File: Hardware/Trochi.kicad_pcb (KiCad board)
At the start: 2 copper layers, 18.5 x 25 mm, 51 parts, among them IC1 ICM-42688-P, J1 JST-SH, J2 JST-SH, J3 JST PH, J6 JST-SH, J7 JST-SH, Q1 AO3400A, Q2 AO3400A, Q3 AO3400A, Q4 AO3400A, Q5 AO3400A, U1 ME6211C33M5, U3 YX-SMD5020

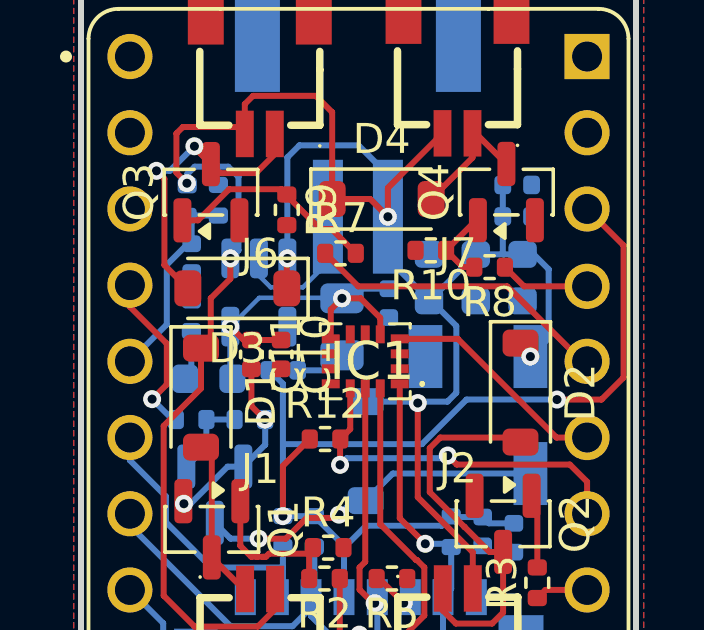
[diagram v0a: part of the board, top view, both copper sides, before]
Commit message: chore: snapshot PCB state before full re-layout
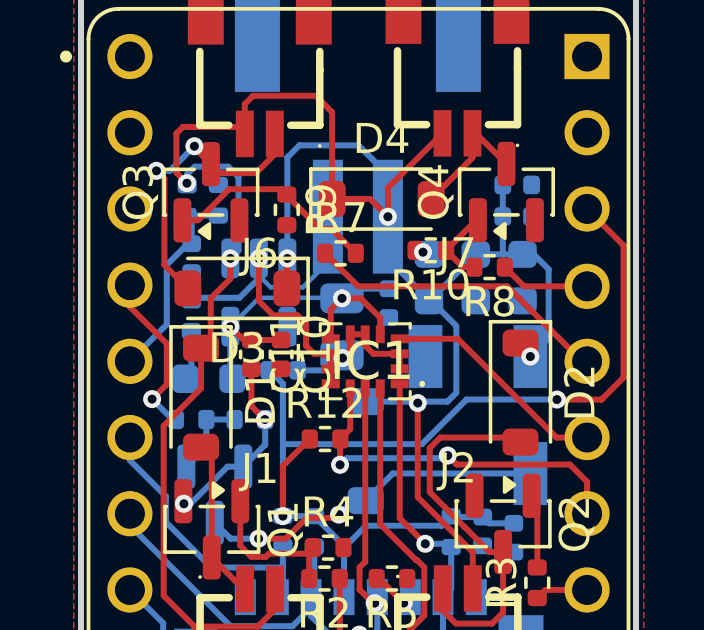
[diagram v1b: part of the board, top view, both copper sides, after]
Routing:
- net GND: track 15.0 -> 28.0 mm, vias 3 -> 6
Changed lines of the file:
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@@
 		(embedded_fonts no)
 		(model "C:/Users/husey/OneDrive/Belgeler/Trochi/Libraries/3D_Models/esp32_s3_supermini.step"
-			(opacity 0.0000)
 			(offset
 				(xyz 0 0 17.5)
@@
 	)
 	(segment
+		(start 139.76 104.33)
+		(end 138.956304 104.33)
+		(width 0.2)
+		(layer "F.Cu")
+		(net "GND")
+	)
+	(segment
+		(start 140.87 105.61)
+		(end 140.32 105.61)
+		(width 0.2)
+		(layer "F.Cu")
+		(net "GND")
+	)
+	(segment
 		(start 142.480947 113.1)
 		(end 143.300947 113.92)
@@
 	)
 	(segment
+		(start 140.87 106.11)
+		(end 140.87 106.61)
+		(width 0.2)
+		(layer "F.Cu")
+		(net "GND")
+	)
+	(segment
+		(start 142.29 105.61)
+		(end 142.02 105.34)
+		(width 0.2)
+		(layer "F.Cu")
+		(net "GND")
+	)
+	(segment
+		(start 143.17 105.61)
+		(end 143.17 106.11)
+		(width 0.2)
+		(layer "F.Cu")
+		(net "GND")
+	)
+	(segment
+		(start 140.32 105.61)
+		(end 140.05 105.34)
+		(width 0.2)
+		(layer "F.Cu")
+		(net "GND")
+	)
+	(segment
 		(start 142.4 113.1)
 		(end 142.480947 113.1)
@@
 	)
 	(segment
+		(start 142.02 104.96)
+		(end 141.52 104.96)
+		(width 0.2)
+		(layer "F.Cu")
+		(net "GND")
+	)
+	(segment
+		(start 140.05 105.34)
+		(end 140.05 104.62)
+		(width 0.2)
+		(layer "F.Cu")
+		(net "GND")
+	)
+	(segment
+		(start 143.17 105.61)
+		(end 142.29 105.61)
+		(width 0.2)
+		(layer "F.Cu")
+		(net "GND")
+	)
+	(segment
+		(start 143.945 102.220865)
+		(end 143.884135 102.16)
+		(width 0.2)
+		(layer "F.Cu")
+		(net "GND")
+	)
+	(segment
+		(start 141.52 105.493583)
+		(end 141.262145 105.751438)
+		(width 0.2)
+		(layer "F.Cu")
+		(net "GND")
+	)
+	(segment
+		(start 140.87 105.61)
+		(end 140.87 106.11)
+		(width 0.2)
+		(layer "F.Cu")
+		(net "GND")
+	)
+	(segment
+		(start 138.956304 104.33)
+		(end 138.475 103.848696)
+		(width 0.2)
+		(layer "F.Cu")
+		(net "GND")
+	)
+	(segment
+		(start 138.475 103.848696)
+		(end 138.475 102.43)
+		(width 0.2)
+		(layer "F.Cu")
+		(net "GND")
+	)
+	(segment
 		(start 138.225 106.11)
 		(end 138.225 107.35)
@@
 	)
 	(segment
+		(start 143.884135 102.16)
+		(end 143.695 102.16)
+		(width 0.2)
+		(layer "F.Cu")
+		(net "GND")
+	)
+	(segment
+		(start 140.05 104.62)
+		(end 139.76 104.33)
+		(width 0.2)
+		(layer "F.Cu")
+		(net "GND")
+	)
+	(segment
 		(start 138.225 107.35)
 		(end 138.675 107.8)
@@
 		(net "GND")
 	)
+	(segment
+		(start 141.52 104.96)
+		(end 141.52 105.493583)
+		(width 0.2)
+		(layer "F.Cu")
+		(net "GND")
+	)
+	(segment
+		(start 142.02 105.34)
+		(end 142.02 104.96)
+		(width 0.2)
+		(layer "F.Cu")
+		(net "GND")
+	)
 	(via
 		(at 138.675 107.8)
@@
 		(net "GND")
 	)
+	(via
+		(at 141.262145 105.751438)
+		(size 0.6)
+		(drill 0.3)
+		(layers "F.Cu" "B.Cu")
+		(net "GND")
+	)
+	(via
+		(at 143.945 102.220865)
+		(size 0.6)
+		(drill 0.3)
+		(layers "F.Cu" "B.Cu")
+		(net "GND")
+	)
+	(via
+		(at 138.475 102.43)
+		(size 0.6)
+		(drill 0.3)
+		(layers "F.Cu" "B.Cu")
+		(net "GND")
+	)
 	(segment
 		(start 140.895 101.19)
@@
 	)
 	(segment
+		(start 138.475 103.092499)
+		(end 138.475 102.43)
+		(width 0.2)
+		(layer "B.Cu")
+		(net "GND")
+	)
+	(segment
 		(start 140.745 106.16)
 		(end 141.245 105.66)
@@
 	)
 	(segment
+		(start 136.225 103.83)
+		(end 136.3125 103.7425)
+		(width 0.2)
+		(layer "B.Cu")
+		(net "GND")
+	)
+	(segment
 		(start 139.9425 103.3925)
 		(end 138.8675 103.3925)
@@
 	)
 	(segment
+		(start 137.824999 103.7425)
+		(end 138.475 103.092499)
+		(width 0.2)
+		(layer "B.Cu")
+		(net "GND")
+	)
+	(segment
 		(start 136.235 103.82)
 		(end 136.225 103.83)
@@
 	)
 	(segment
+		(start 136.3125 103.7425)
+		(end 137.824999 103.7425)
+		(width 0.2)
+		(layer "B.Cu")
+		(net "GND")
+	)
+	(segment
 		(start 138.685 107.8)
 		(end 138.685 108.64)
@@
 		(hatch edge 0.5)
 		(connect_pads
-			(clearance 0.3)
+			(clearance 0.2)
 		)
 		(min_thickness 0.25)

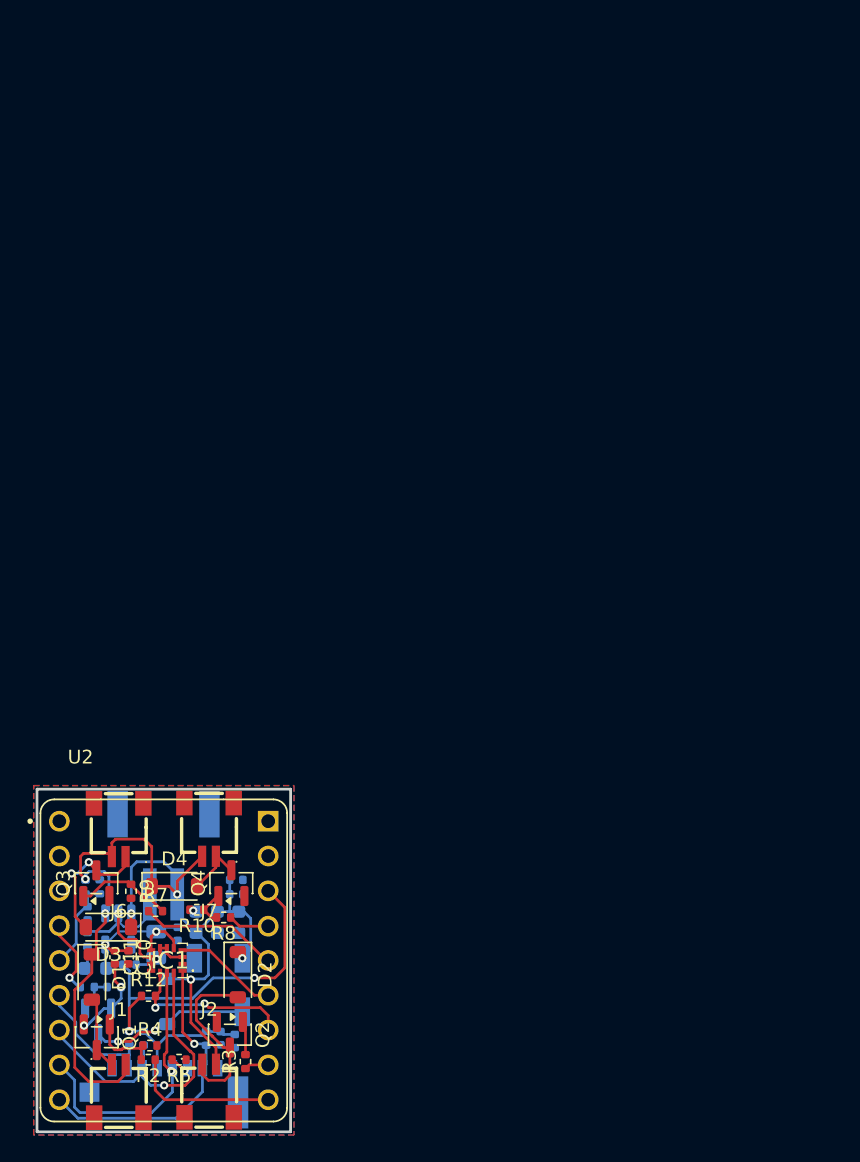
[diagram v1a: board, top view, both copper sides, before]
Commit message: feat: Routing Completed :)
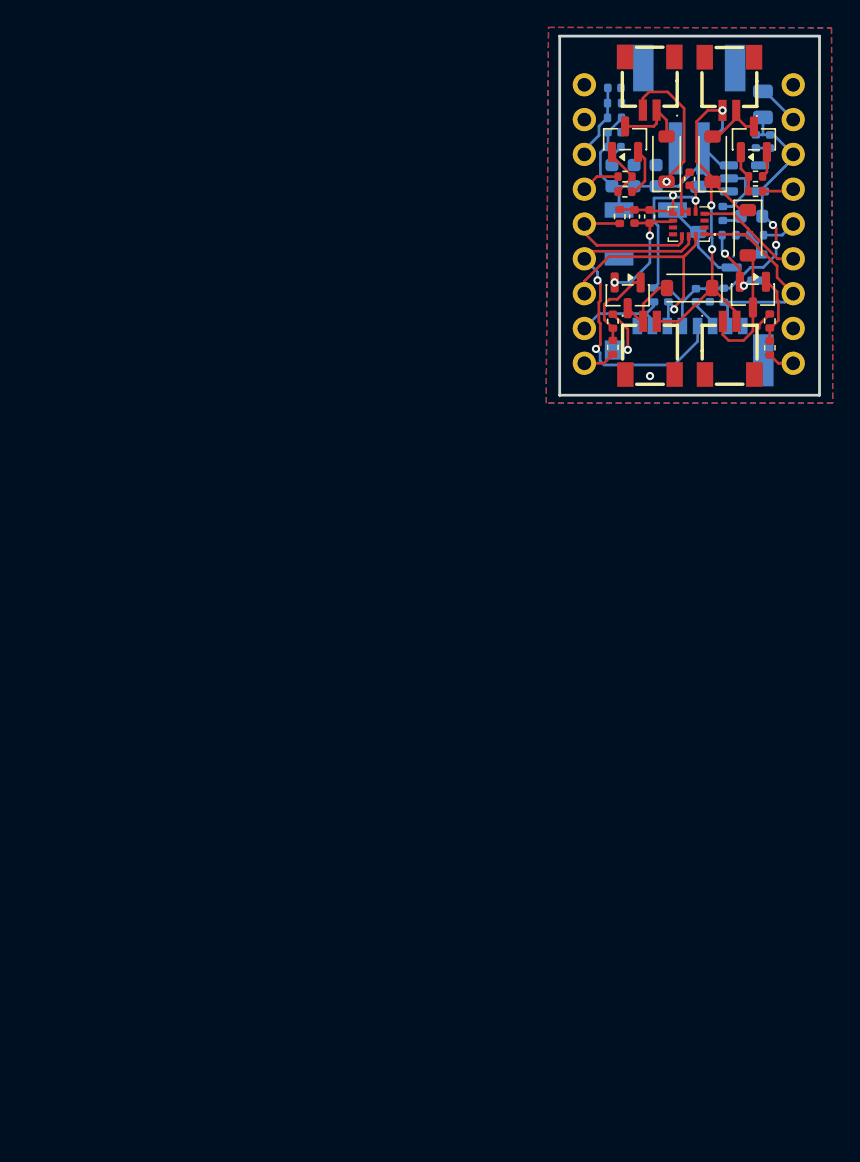
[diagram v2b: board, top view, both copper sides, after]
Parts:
- removed U2: ~, trochi_footprint:esp32_s3_supermini
- added C14: 10nF, Capacitor_SMD:C_0402_1005Metric, F.Cu at (176.1, 51.6)
- added J4: Conn_01x09, Connector_PinHeader_2.54mm:PinHeader_1x09_P2.54mm_Vertical, F.Cu at (172.5, 42.0)
- added J5: Conn_01x09, Connector_PinHeader_2.54mm:PinHeader_1x09_P2.54mm_Vertical, F.Cu at (187.7, 42.0)
- C11: value 100nF -> 2.2uF
- moved C6 75.6 mm to (185.5, 43.4), turned to 90 degrees
- moved C7 75.5 mm to (185.0, 46.1), turned to -90 degrees
- moved R16 73.4 mm to (185.0, 52.9), turned to 180 degrees
- moved D5 72.8 mm to (184.7, 51.6)
- moved Q5 72.5 mm to (184.2, 55.3), turned to 180 degrees
- moved C8 72.2 mm to (186.0, 46.1)
- moved C9 71.4 mm to (174.7, 42.2), turned to 0 degrees
- moved U1 71.3 mm to (184.2, 48.8), turned to 0 degrees
- moved R17 70.9 mm to (183.0, 52.9), turned to 180 degrees
- moved R11 70.4 mm to (182.6, 51.4)
- moved C10 70.0 mm to (180.2, 48.8)
- moved D6 69.6 mm to (180.8, 51.1)
- moved D3 69.3 mm to (178.5, 47.4), turned to 90 degrees
- moved R5 69.0 mm to (186.0, 59.2), turned to 90 degrees
- moved R6 68.4 mm to (174.7, 43.3), turned to 0 degrees
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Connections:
- C10 pad 1: +3.3V -> GND
- C10 pad 2: GND -> +3.3V
- C11 pad 1: +3.3V -> GND
- C11 pad 2: GND -> +3.3V
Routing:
- net GND: track 28.0 -> 41.2 mm
- net /VBAT: track 77.0 -> 68.4 mm, vias 6 -> 4
- net +3.3V: track 51.4 -> 43.6 mm
- net PWM_M1: track 10.8 -> 3.03 mm
- net PWM_M3: track 10.2 -> 2.84 mm
- net SPI_MISO: track 21.9 -> 15.9 mm, vias 1 -> 0
- net SPI_SCK: track 20.7 -> 26.3 mm, vias 1 -> 2
- net Net-(D6-A): track 11.6 -> 6.70 mm, vias 2 -> 0
- net SPI_MOSI: track 23.3 -> 18.4 mm
- net Net-(D3-A): track 9.97 -> 5.58 mm, vias 2 -> 0
- net Net-(D2-A): track 13.1 -> 9.32 mm
- net Net-(Q3-G): track 7.12 -> 3.92 mm
- net BUZZER_CTRL: track 5.58 -> 2.50 mm, vias 1 -> 0
- net Net-(Q2-G): track 2.47 -> 5.03 mm
- net CS_SD: track 9.59 -> 7.42 mm
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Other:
- board size 18.5 x 25 mm -> 19 x 26.2 mm
